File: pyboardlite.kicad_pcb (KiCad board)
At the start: 2 copper layers, 35.6 x 26.4 mm, 30 parts, among them J1 USB_OTG, J2 Conn_02x03_Odd_Even, SW1 Button-PTM, U1 LP2980AIM5-3.3, U2 STM32F405RGT6, Y1 8MHz

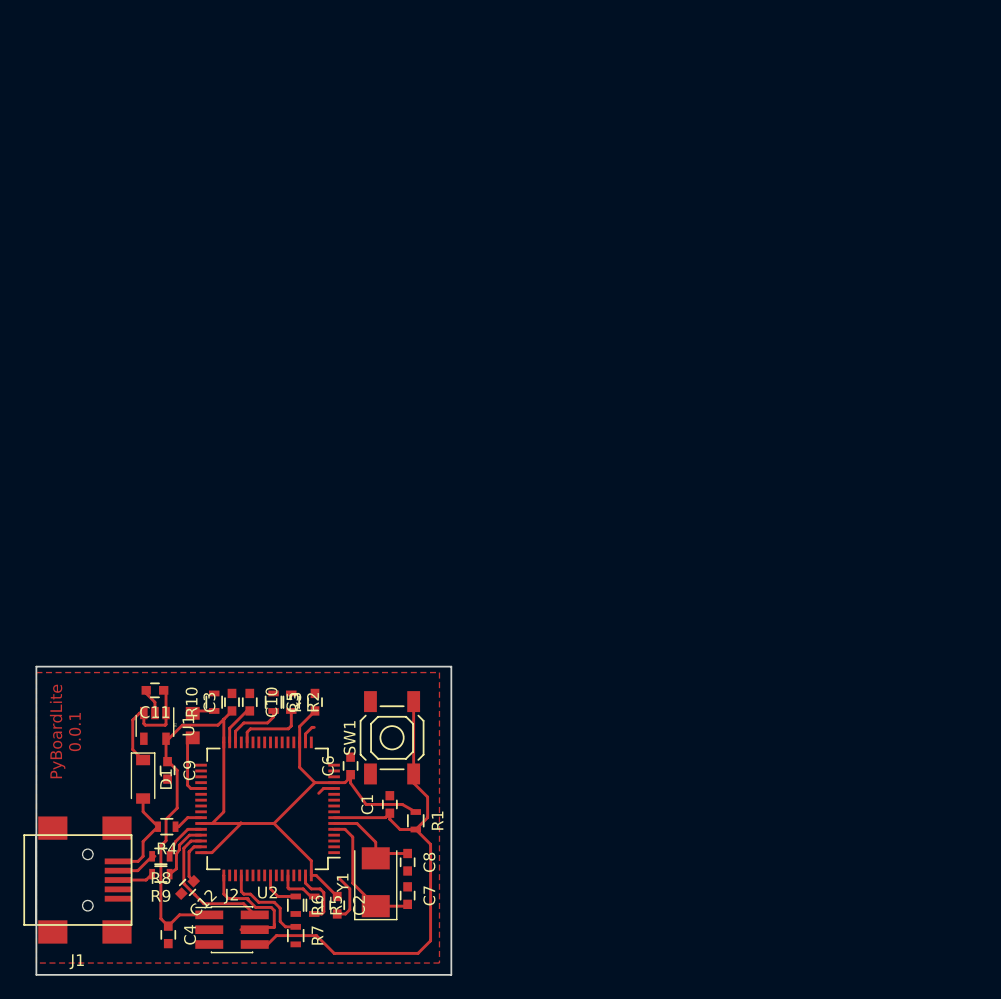
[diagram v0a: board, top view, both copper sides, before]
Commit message: Jiggery pokery
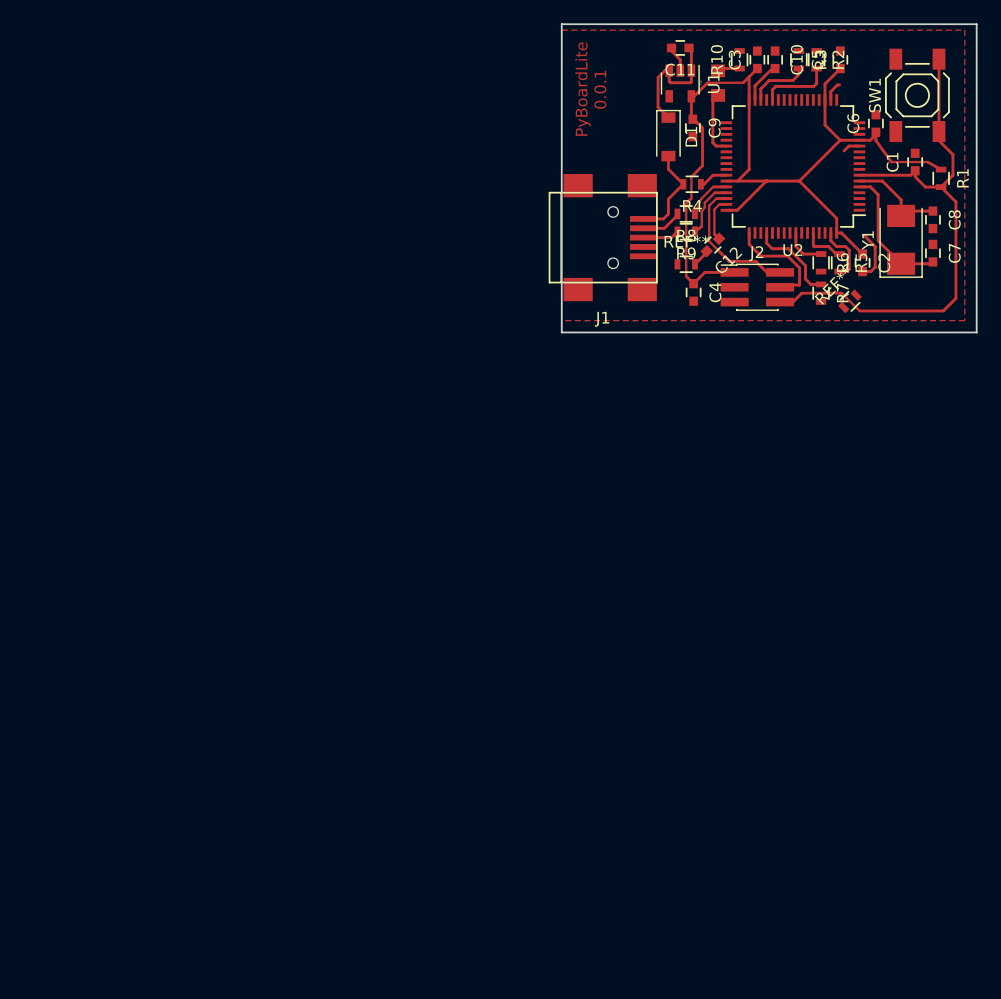
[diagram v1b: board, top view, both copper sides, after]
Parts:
- added REF**: R_0603, Resistors_SMD:R_0603, F.Cu at (264.3, 46.9)
- added REF**: R_0603, Resistors_SMD:R_0603, F.Cu at (250.3, 43.8)
- moved R2 71.1 mm to (261.4, 26.2)
- moved R3 71.1 mm to (259.9, 26.2)
- moved R5 71.1 mm to (263.4, 43.6)
- moved C1 71.1 mm to (269.9, 35.0)
- moved C12 71.1 mm to (252.5, 42.1)
- moved C5 71.1 mm to (263.5, 26.2)
- moved C6 71.1 mm to (266.5, 31.7)
- moved D2 71.1 mm to (253.0, 27.2)
- moved R1 71.1 mm to (272.1, 36.4)
- moved R10 71.1 mm to (254.8, 26.2)
- moved R6 71.1 mm to (261.8, 43.6)
- moved C11 71.1 mm to (249.7, 25.2)
- moved C4 71.1 mm to (250.9, 46.2)
- moved C7 71.1 mm to (271.4, 42.8)
- moved C8 71.1 mm to (271.4, 39.9)
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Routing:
- net /SWCLK: track 11.0 -> 9.34 mm
- net GND: track 14.8 -> 16.4 mm
